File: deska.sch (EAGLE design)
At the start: 25 parts, among them Q1 BC547, X1 JST-XH-03-PIN-LONG-PAD, X2 JST-XH-03-PIN-LONG-PAD, X3 JST-XH-03-PIN-LONG-PAD, X4 JST-XH-04-PIN-LONG-PAD, X5 JST-XH-04-PIN-LONG-PAD, X6 JST-XH-04-PIN-LONG-PAD

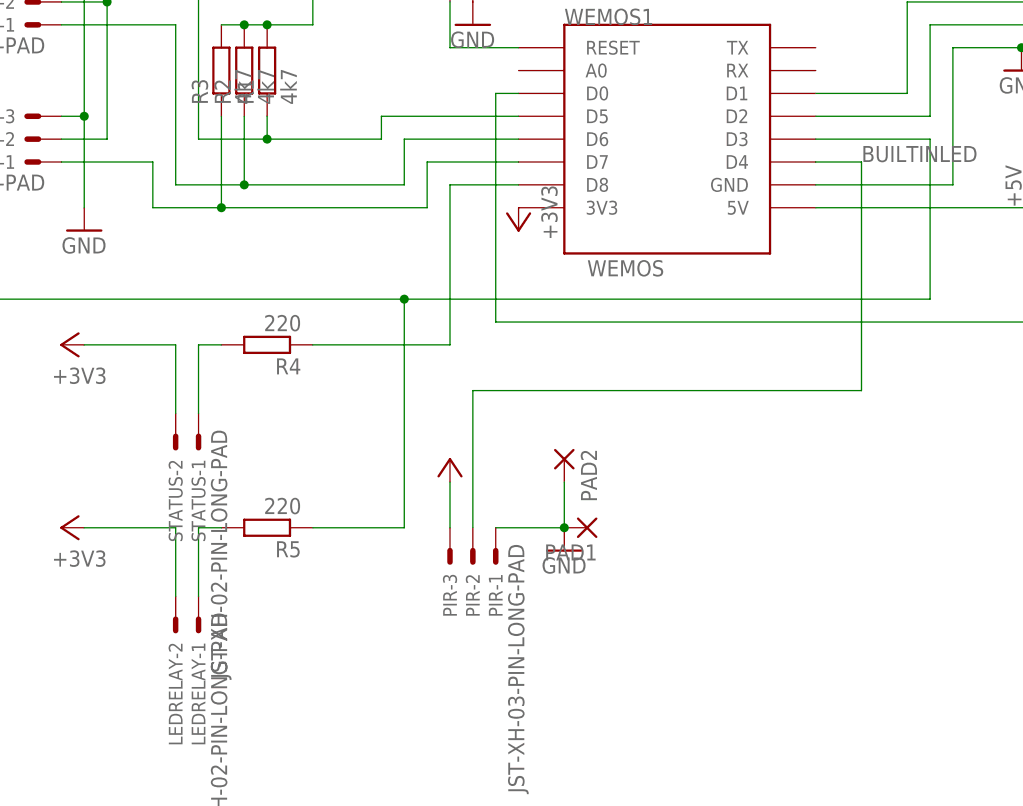
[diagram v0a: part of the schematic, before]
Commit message: +
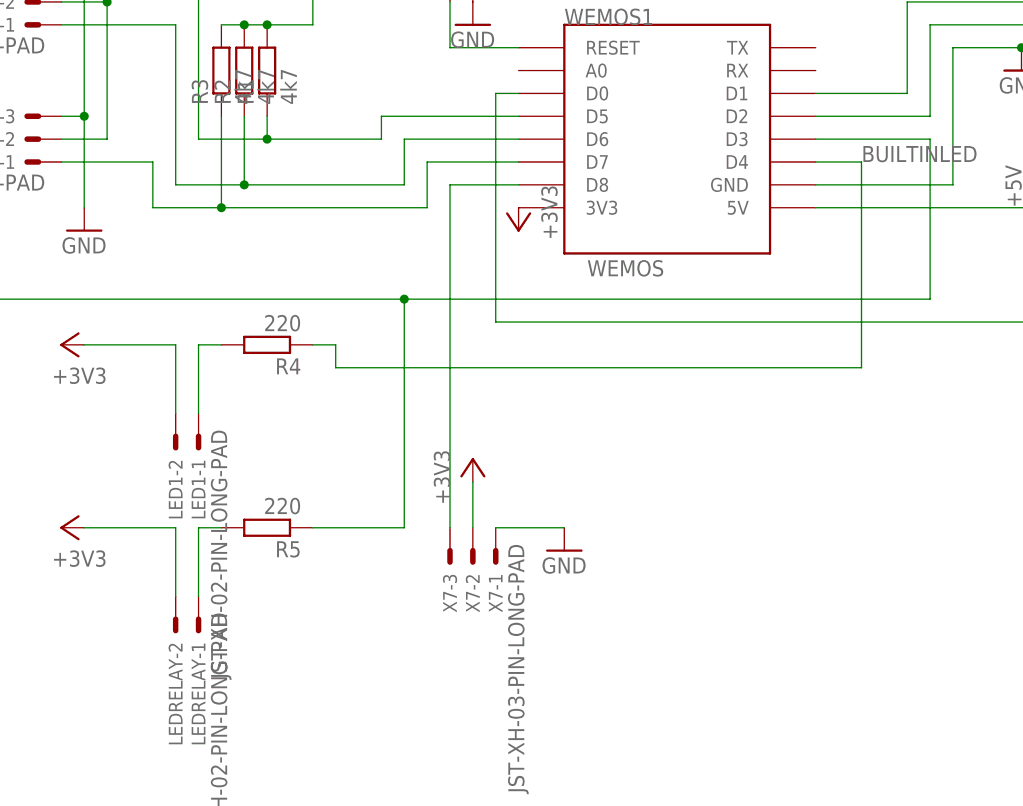
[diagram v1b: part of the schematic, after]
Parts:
- removed PAD1, PAD2: (no value), wirepad:2,15/1,0
- renumbered PIR to X7, STATUS to LED1
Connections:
- net +3V3: now also X7-2.S; no longer X7-3.S
- net BUILTINLED: now also WEMOS1.D4; no longer WEMOS1.D8
- net GND: no longer PAD1.P, PAD2.P
- net N$3: now also WEMOS1.D8, X7-3.S; no longer WEMOS1.D4, X7-2.S
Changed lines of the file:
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@@
 <part name="X6" library="Rembrandt Electronics - JST XH Connectors v1-0" deviceset="JST-XH-04-PIN" device="-LONG-PAD"/>
 <part name="RELAY" library="Rembrandt Electronics - JST XH Connectors v1-0" deviceset="JST-XH-03-PIN" device="-LONG-PAD"/>
-<part name="STATUS" library="Rembrandt Electronics - JST XH Connectors v1-0" deviceset="JST-XH-02-PIN" device="-LONG-PAD"/>
+<part name="LED1" library="Rembrandt Electronics - JST XH Connectors v1-0" deviceset="JST-XH-02-PIN" device="-LONG-PAD"/>
 <part name="LEDRELAY" library="Rembrandt Electronics - JST XH Connectors v1-0" deviceset="JST-XH-02-PIN" device="-LONG-PAD"/>
 <part name="BUZZER" library="Rembrandt Electronics - JST XH Connectors v1-0" deviceset="JST-XH-02-PIN" device="-LONG-PAD"/>
@@
 <part name="GND2" library="supply1" deviceset="GND" device=""/>
 <part name="+3V5" library="supply1" library_urn="urn:adsk.eagle:library:371" deviceset="+3V3" device=""/>
-<part name="PIR" library="Rembrandt Electronics - JST XH Connectors v1-0" deviceset="JST-XH-03-PIN" device="-LONG-PAD"/>
+<part name="X7" library="Rembrandt Electronics - JST XH Connectors v1-0" deviceset="JST-XH-03-PIN" device="-LONG-PAD"/>
 <part name="GND3" library="supply1" deviceset="GND" device=""/>
 <part name="RESET" library="Rembrandt Electronics - JST XH Connectors v1-0" deviceset="JST-XH-02-PIN" device="-LONG-PAD"/>
 <part name="GND7" library="supply1" deviceset="GND" device=""/>
-<part name="PAD1" library="wirepad" library_urn="urn:adsk.eagle:library:412" deviceset="2,15/1,0" device="" package3d_urn="urn:adsk.eagle:package:30831/1"/>
-<part name="PAD2" library="wirepad" library_urn="urn:adsk.eagle:library:412" deviceset="2,15/1,0" device="" package3d_urn="urn:adsk.eagle:package:30831/1"/>
 </parts>
 <sheets>
@@
 <attribute name="NAME" x="-33.02" y="56.642" size="1.524" layer="95" rot="R180"/>
 </instance>
-<instance part="STATUS" gate="-2" x="10.16" y="27.94" smashed="yes" rot="R270">
+<instance part="LED1" gate="-2" x="10.16" y="27.94" smashed="yes" rot="R270">
 <attribute name="NAME" x="9.398" y="25.4" size="1.524" layer="95" rot="R270"/>
 </instance>
-<instance part="STATUS" gate="-1" x="12.7" y="27.94" smashed="yes" rot="R270">
+<instance part="LED1" gate="-1" x="12.7" y="27.94" smashed="yes" rot="R270">
 <attribute name="NAME" x="11.938" y="25.4" size="1.524" layer="95" rot="R270"/>
 <attribute name="VALUE" x="14.097" y="28.702" size="1.778" layer="96" rot="R270"/>
@@
 <attribute name="VALUE" x="101.6" y="66.04" size="1.778" layer="96"/>
 </instance>
-<instance part="+3V5" gate="G$1" x="40.64" y="25.4" smashed="yes"/>
-<instance part="PIR" gate="-1" x="45.72" y="15.24" smashed="yes" rot="R270">
+<instance part="+3V5" gate="G$1" x="43.18" y="25.4" smashed="yes">
+<attribute name="VALUE" x="40.64" y="20.32" size="1.778" layer="96" rot="R90"/>
+</instance>
+<instance part="X7" gate="-1" x="45.72" y="15.24" smashed="yes" rot="R270">
 <attribute name="NAME" x="44.958" y="12.7" size="1.524" layer="95" rot="R270"/>
 <attribute name="VALUE" x="47.117" y="16.002" size="1.778" layer="96" rot="R270"/>
 </instance>
-<instance part="PIR" gate="-2" x="43.18" y="15.24" smashed="yes" rot="R270">
+<instance part="X7" gate="-2" x="43.18" y="15.24" smashed="yes" rot="R270">
 <attribute name="NAME" x="42.418" y="12.7" size="1.524" layer="95" rot="R270"/>
 </instance>
-<instance part="PIR" gate="-3" x="40.64" y="15.24" smashed="yes" rot="R270">
+<instance part="X7" gate="-3" x="40.64" y="15.24" smashed="yes" rot="R270">
 <attribute name="NAME" x="39.878" y="12.7" size="1.524" layer="95" rot="R270"/>
 </instance>
@@
 <instance part="GND7" gate="1" x="43.18" y="73.66" smashed="yes">
 <attribute name="VALUE" x="40.64" y="71.12" size="1.778" layer="96"/>
-</instance>
-<instance part="PAD1" gate="1" x="55.88" y="17.78" smashed="yes" rot="R180">
-<attribute name="NAME" x="57.023" y="15.9258" size="1.778" layer="95" rot="R180"/>
-<attribute name="VALUE" x="57.023" y="21.082" size="1.778" layer="96" rot="R180"/>
-</instance>
-<instance part="PAD2" gate="1" x="53.34" y="25.4" smashed="yes" rot="R270">
-<attribute name="NAME" x="55.1942" y="26.543" size="1.778" layer="95" rot="R270"/>
-<attribute name="VALUE" x="50.038" y="26.543" size="1.778" layer="96" rot="R270"/>
 </instance>
 </instances>
@@
 </segment>
 <segment>
+<pinref part="X7" gate="-1" pin="S"/>
 <pinref part="GND3" gate="1" pin="GND"/>
-<pinref part="PAD1" gate="1" pin="P"/>
-<pinref part="PIR" gate="-1" pin="S"/>
 <wire x1="45.72" y1="17.78" x2="53.34" y2="17.78" width="0.1524" layer="91"/>
-<junction x="53.34" y="17.78"/>
-<pinref part="PAD2" gate="1" pin="P"/>
-<wire x1="53.34" y1="22.86" x2="53.34" y2="17.78" width="0.1524" layer="91"/>
 </segment>
 <segment>
@@
 <pinref part="R4" gate="G$1" pin="2"/>
 <wire x1="12.7" y1="38.1" x2="15.24" y2="38.1" width="0.1524" layer="91"/>
-<pinref part="STATUS" gate="-1" pin="S"/>
+<pinref part="LED1" gate="-1" pin="S"/>
 <wire x1="12.7" y1="30.48" x2="12.7" y2="38.1" width="0.1524" layer="91"/>
 </segment>
@@
 <net name="BUILTINLED" class="0">
 <segment>
+<pinref part="WEMOS1" gate="D1" pin="D4"/>
+<wire x1="81.28" y1="58.42" x2="86.36" y2="58.42" width="0.1524" layer="91"/>
 <label x="86.36" y="58.42" size="1.778" layer="95"/>
+<wire x1="86.36" y1="58.42" x2="86.36" y2="35.56" width="0.1524" layer="91"/>
+<wire x1="27.94" y1="38.1" x2="25.4" y2="38.1" width="0.1524" layer="91"/>
 <pinref part="R4" gate="G$1" pin="1"/>
-<wire x1="25.4" y1="38.1" x2="40.64" y2="38.1" width="0.1524" layer="91"/>
-<wire x1="40.64" y1="38.1" x2="40.64" y2="55.88" width="0.1524" layer="91"/>
-<pinref part="WEMOS1" gate="D1" pin="D8"/>
-<wire x1="40.64" y1="55.88" x2="48.26" y2="55.88" width="0.1524" layer="91"/>
+<wire x1="86.36" y1="35.56" x2="27.94" y2="35.56" width="0.1524" layer="91"/>
+<wire x1="27.94" y1="35.56" x2="27.94" y2="38.1" width="0.1524" layer="91"/>
 </segment>
 </net>
@@
 <pinref part="+3V2" gate="G$1" pin="+3V3"/>
 <wire x1="10.16" y1="38.1" x2="0" y2="38.1" width="0.1524" layer="91"/>
-<pinref part="STATUS" gate="-2" pin="S"/>
+<pinref part="LED1" gate="-2" pin="S"/>
 <wire x1="10.16" y1="38.1" x2="10.16" y2="30.48" width="0.1524" layer="91"/>
 </segment>
@@
 </segment>
 <segment>
-<pinref part="PIR" gate="-3" pin="S"/>
 <pinref part="+3V5" gate="G$1" pin="+3V3"/>
-<wire x1="40.64" y1="17.78" x2="40.64" y2="22.86" width="0.1524" layer="91"/>
+<wire x1="43.18" y1="22.86" x2="43.18" y2="17.78" width="0.1524" layer="91"/>
+<pinref part="X7" gate="-2" pin="S"/>
 </segment>
 </net>
@@
 </segment>
 </net>
+<net name="N$3" class="0">
+<segment>
+<pinref part="WEMOS1" gate="D1" pin="D8"/>
+<wire x1="48.26" y1="55.88" x2="40.64" y2="55.88" width="0.1524" layer="91"/>
+<wire x1="40.64" y1="17.78" x2="40.64" y2="55.88" width="0.1524" layer="91"/>
+<pinref part="X7" gate="-3" pin="S"/>
+</segment>
+</net>
 <net name="N$5" class="0">
 <segment>
@@
 </segment>
 </net>
-<net name="N$3" class="0">
-<segment>
-<wire x1="43.18" y1="33.02" x2="86.36" y2="33.02" width="0.1524" layer="91"/>
-<wire x1="86.36" y1="33.02" x2="86.36" y2="58.42" width="0.1524" layer="91"/>
-<pinref part="WEMOS1" gate="D1" pin="D4"/>
-<wire x1="86.36" y1="58.42" x2="81.28" y2="58.42" width="0.1524" layer="91"/>
-<pinref part="PIR" gate="-2" pin="S"/>
-<wire x1="43.18" y1="17.78" x2="43.18" y2="33.02" width="0.1524" layer="91"/>
-</segment>
-</net>
